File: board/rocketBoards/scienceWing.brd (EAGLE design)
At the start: 18.7 x 10.5 mm, 10 parts, among them U1 HTU21DSMD

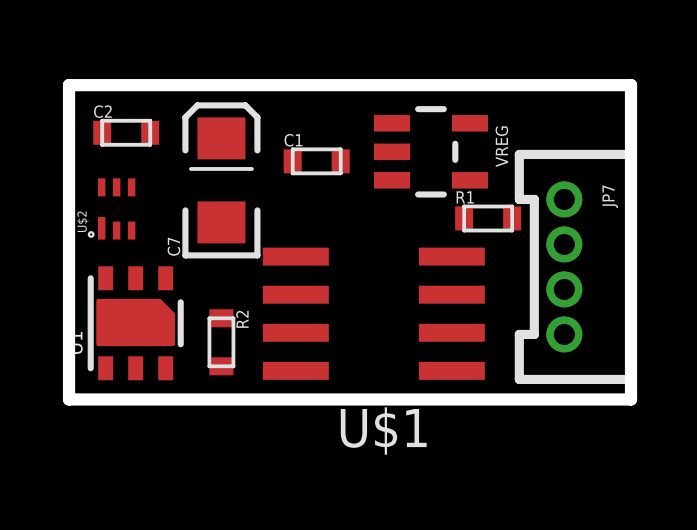
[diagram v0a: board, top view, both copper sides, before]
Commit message: boards shipped
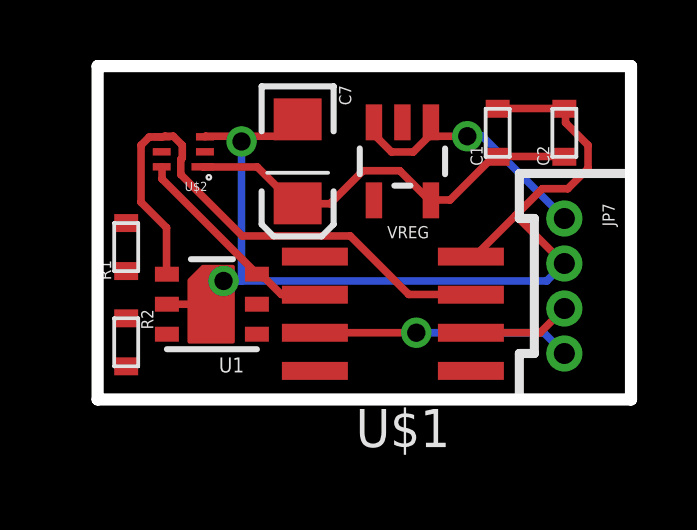
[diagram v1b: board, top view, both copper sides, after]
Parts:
- moved C2 14.6 mm to (16.5, 8.89), turned to 90 degrees
- moved R1 12.1 mm to (1.91, 5.08), turned to 90 degrees
- moved C1 6.11 mm to (14.3, 8.89), turned to 90 degrees
- moved R2 3.17 mm to (1.91, 1.91)
- moved U$2 2.93 mm to (3.81, 8.26), turned to 180 degrees
- moved C7 2.62 mm to (7.62, 7.94), turned to 270 degrees
- moved U1 2.62 mm to (4.76, 3.17), turned to 180 degrees
- moved VREG 1.00 mm to (11.1, 7.94), turned to 180 degrees
- moved JP7 0.64 mm to (16.5, 6.03)
- moved U$1 0.63 mm to (10.8, 2.86)
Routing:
- net GND: track 0.00 -> 34.2 mm, vias 0 -> 2
- net I2C_SDA: track 0.00 -> 18.6 mm
- net VCC: track 0.00 -> 14.1 mm
- net VBATT: track 0.00 -> 9.15 mm, vias 0 -> 1
- net I2CB2B_SCL: track 0.00 -> 8.61 mm, vias 0 -> 1
- net I2C_SCL: track 0.00 -> 7.12 mm
- net I2CB2B_SDA: track 0.00 -> 3.45 mm
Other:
- board size 18.7 x 10.5 mm -> 17.8 x 11.1 mm
